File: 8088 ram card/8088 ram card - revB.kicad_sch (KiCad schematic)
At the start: 40 parts, among them J2 Conn_01x16_Socket, J3 Conn_01x16_Socket, P2 Conn_01x16_Pin, P3 Conn_01x16_Pin, Q1 2N3904, U1 4164, U10 74S04, U11 74S04, U12 74S00, U2 4164, U3 4164, U4 4164, U5 4164, U6 4164, U7 4164, U8 4164, U9 4164

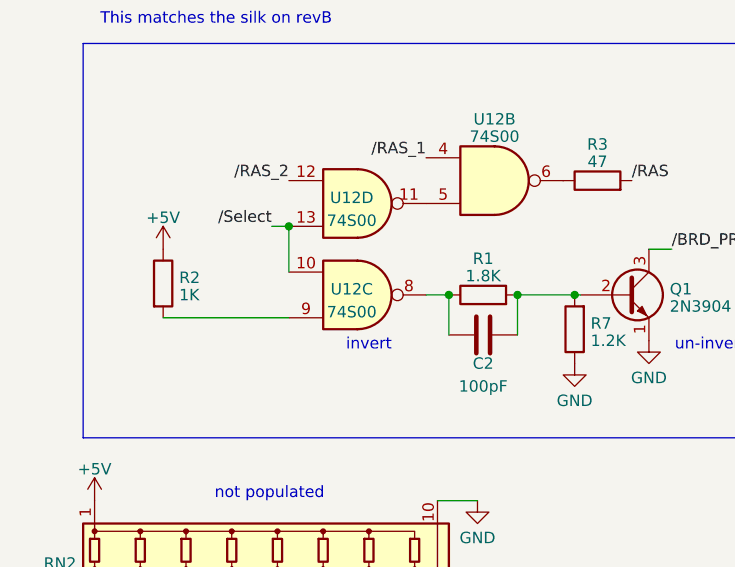
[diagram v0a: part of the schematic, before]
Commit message: finished latest rev ram card version
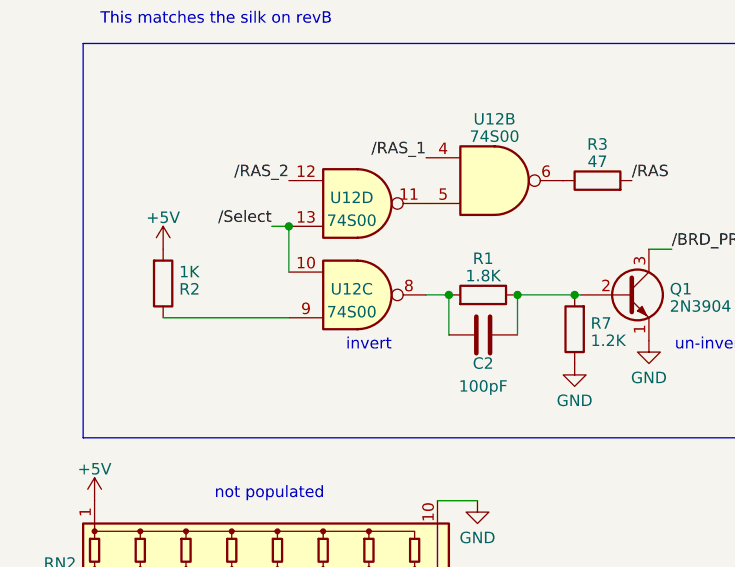
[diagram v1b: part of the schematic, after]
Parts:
- C1: footprint (none) -> Evan's parts:noethstar tantalum
- C10, C11, C12, C13, C14, C2, C3, C4, C5, C6, C7, C8, C9: footprint (none) -> Evan's parts:northstar decoupling cap
- J2: footprint (none) -> Connector_PinSocket_2.54mm:PinSocket_1x16_P2.54mm_Vertical
- J3: footprint (none) -> Connector_PinSocket_2.54mm:PinSocket_1x18_P2.54mm_Vertical
- P2: footprint (none) -> Connector_PinHeader_2.54mm:PinHeader_1x16_P2.54mm_Vertical
- P3: footprint (none) -> Connector_PinHeader_2.54mm:PinHeader_1x18_P2.54mm_Vertical
- Q1: footprint Package_TO_SOT_THT:TO-92_Inline -> Evan's parts:TO-92_northstar_Wide
- R1, R2, R3, R4, R5, R6, R7: footprint (none) -> Evan's parts:northstar resistor
- RN1: footprint (none) -> Package_DIP:DIP-16_W7.62mm
- U1, U2, U3, U4, U5, U6, U7, U8, U9: footprint DIL16 -> Package_DIP:DIP-16_W7.62mm
- U10, U11, U12: footprint (none) -> Package_DIP:DIP-14_W7.62mm
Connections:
- net +5V: now also R2.2; no longer R2.1
- net at Q1.2 (B), R7.2: now also C2.1, R1.1; no longer C2.2, R1.2
- net at U12.9: now also R2.1; no longer R2.2
- new net: C2.2, R1.2, U12.8
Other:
- moved on the sheet: C2, R1
